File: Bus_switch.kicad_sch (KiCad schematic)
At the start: 15 parts, among them J3 Conn_01x04_Pin, U1 SN74CB3Q3245PWR

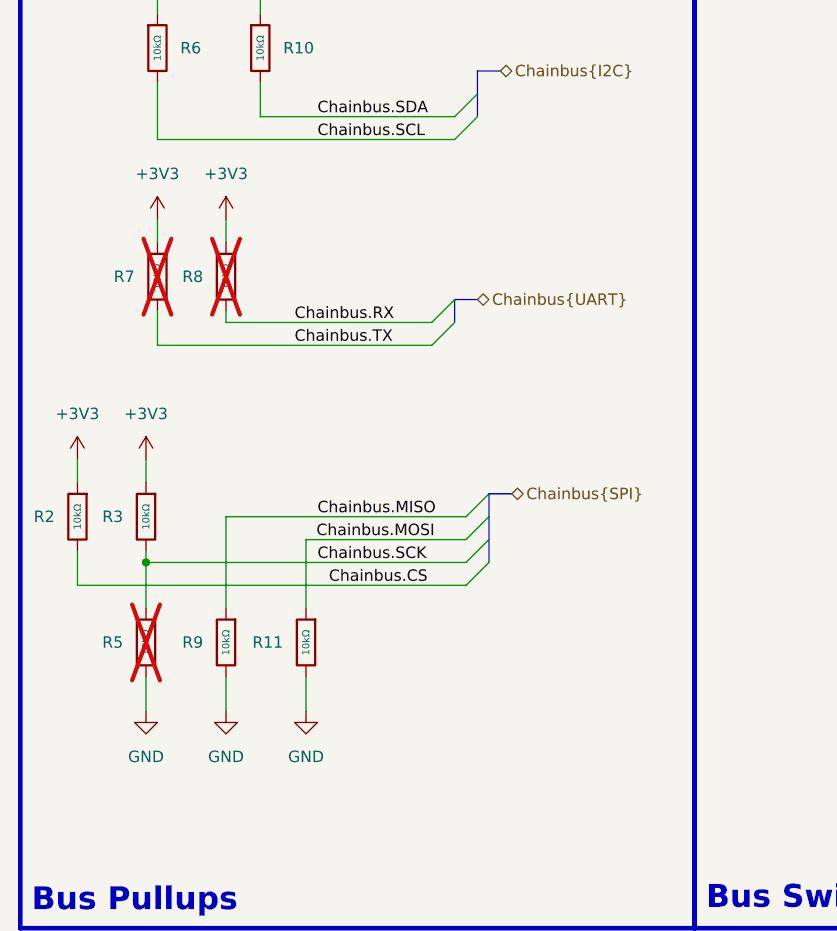
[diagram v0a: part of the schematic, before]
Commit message: inital layout
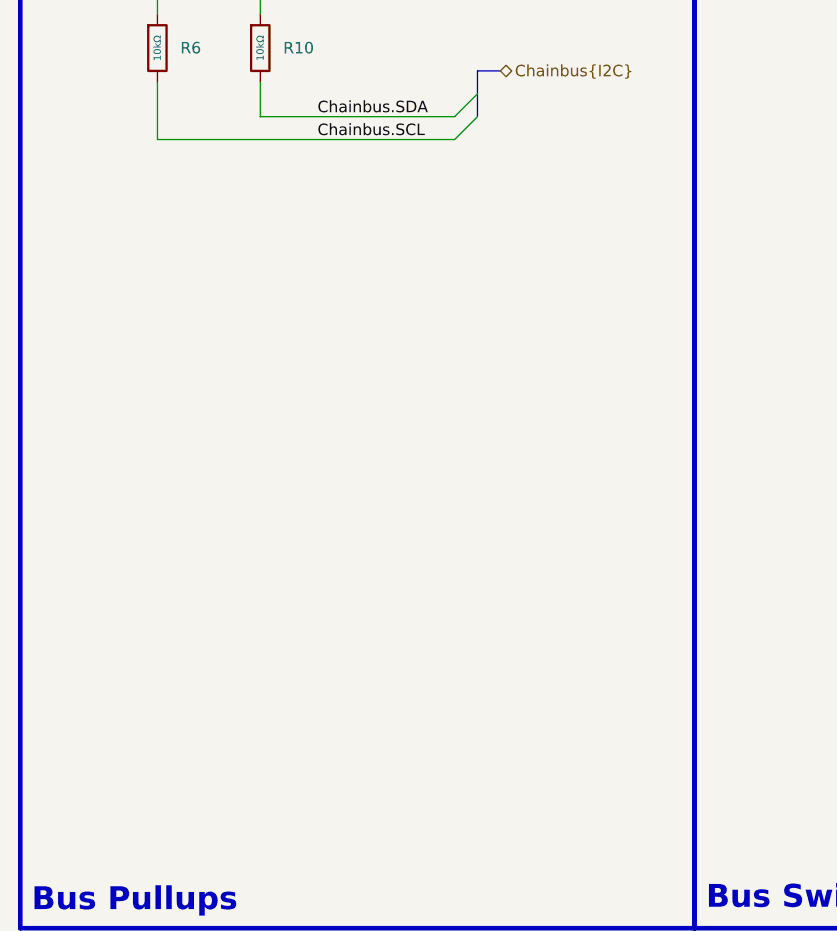
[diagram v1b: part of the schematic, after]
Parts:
- removed R11, R2, R3, R5, R7, R8, R9: 10kΩ, PCM_JLCPCB:R_0402, symbol PCM_JLCPCB-Resistors:0402,10kΩ
